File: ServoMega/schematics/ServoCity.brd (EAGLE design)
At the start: 108.9 x 55.9 mm, 2 parts

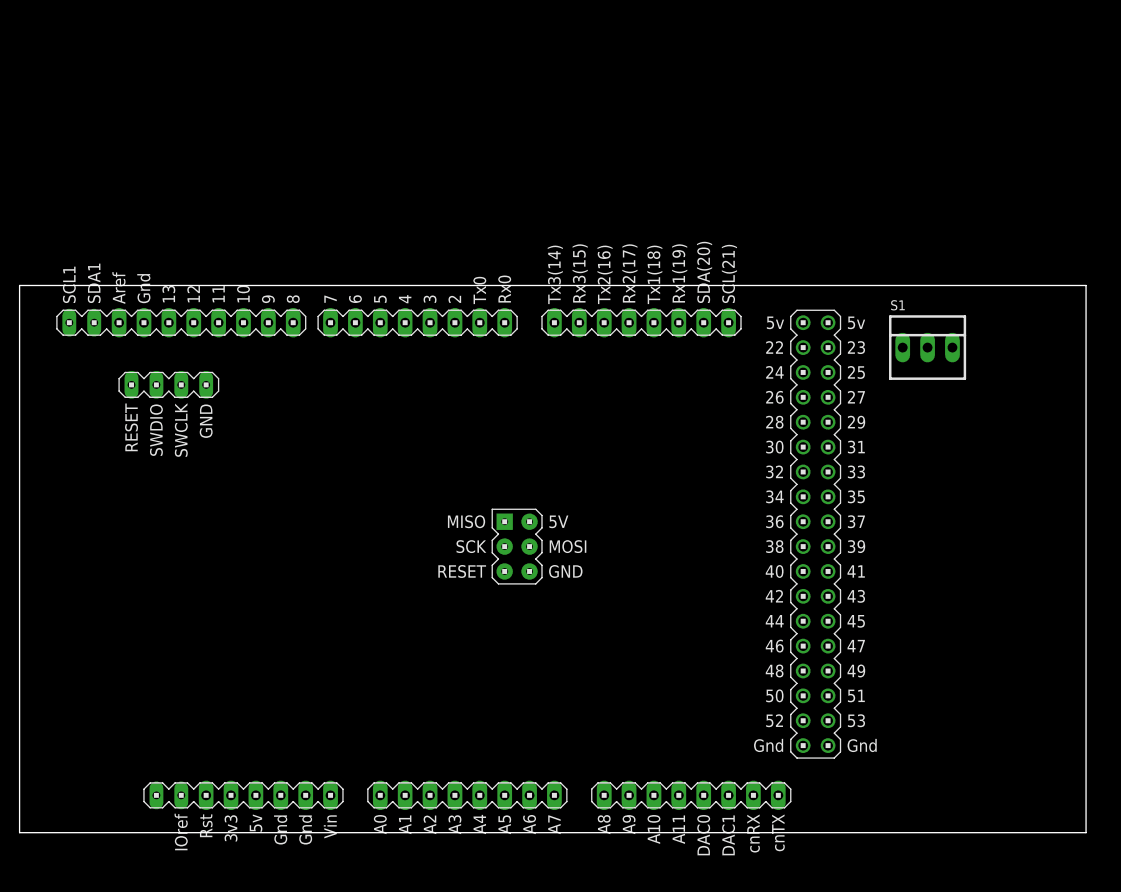
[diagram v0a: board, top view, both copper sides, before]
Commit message: HOK post laptop update
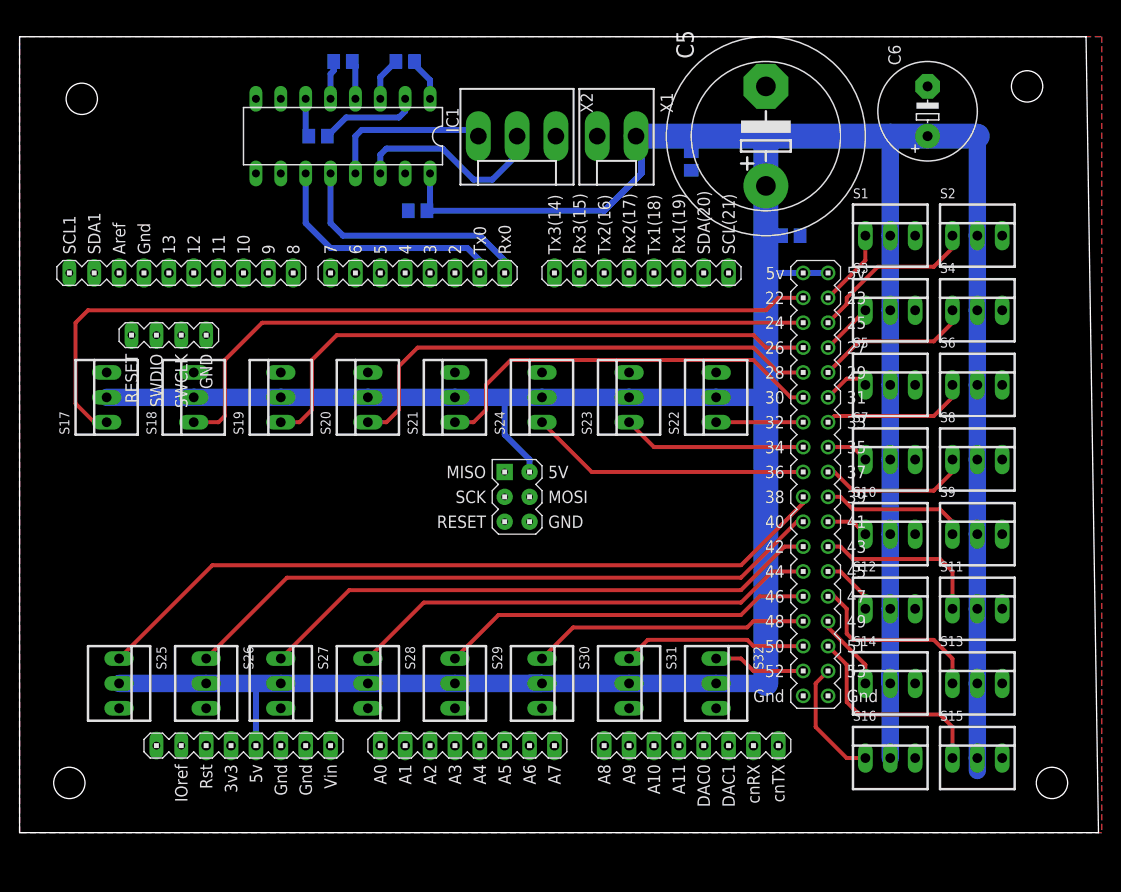
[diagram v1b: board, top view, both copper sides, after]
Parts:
- added C1, C2, C3, C4: (no value), rcl:C0805
- added C5: 2k2, rcl:EB20D
- added C6: 470, rcl:E5-10,5
- added C8, C9: (no value), eagle-ltspice:C0805
- added IC1: MAX232, maxim:DIL16
- added S10, S11, S12, S13, S14, S15, S16, S17, S18, S19, S2, S20, S21, S22, S23, S24, S25, S26, S27, S28, S29, S3, S30, S31, S32, S4, S5, S6, S7, S8, S9: 22-23-2031, con-molex:22-23-2031
- added X1: (no value), con-molex:KK-156-2
- added X2: (no value), con-molex:KK-156-3
- moved S1 12.0 mm to (88.9, 61.0)
- moved U$1 5.08 mm to (61.0, 26.7)
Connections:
- new net 5V: C5.+, C6.+, C8.1, C9.1, S1.2, S10.2, S11.2, S12.2, S13.2, S14.2, S15.2, S16.2, S17.2, S18.2, S19.2, S2.2, S20.2, S21.2, S22.2, S23.2, S24.2, S25.2, S26.2, S27.2, S28.2, S29.2, S3.2, S30.2, S31.2, S32.2, S4.2, S5.2, S6.2, S7.2, S8.2, S9.2, X1.1
- new net GND: C4.2, C5.-, C6.-, C8.2, C9.2, IC1.15, S1.3, S10.3, S11.3, S12.3, S13.3, S14.3, S15.3, S16.3, S17.3, S18.3, S19.3, S2.3, S20.3, S21.3, S22.3, S23.3, S24.3, S25.3, S26.3, S27.3, S28.3, S29.3, S3.3, S30.3, S31.3, S32.3, S4.3, S5.3, S6.3, S7.3, S8.3, S9.3, U$1.5V_ICSP, U$1.GND1, U$1.GND_1, U$1.GND_2, U$1.GND_A, U$1.GND_B, X1.2, X2.1
- new net N$1: IC1.14, X2.2
- new net N$2: IC1.13, X2.3
- new net N$3: C1.1, IC1.1
- new net N$4: C1.2, IC1.3
- new net N$5: C2.1, IC1.4
- new net N$6: C2.2, IC1.5
- new net N$7: C3.1, IC1.2
- new net N$8: C3.2, IC1.6
- new net RX: IC1.12, U$1.RX0
- new net SERVO1: S1.1, U$1.23
- new net SERVO10: S10.1, U$1.41
- new net SERVO11: S11.1, U$1.43
- new net SERVO12: S12.1, U$1.45
- new net SERVO13: S13.1, U$1.47
- new net SERVO14: S14.1, U$1.49
- new net SERVO15: S15.1, U$1.51
- new net SERVO16: S16.1, U$1.53
- new net SERVO17: S17.1, U$1.22
- new net SERVO18: S18.1, U$1.24
- new net SERVO19: S19.1, U$1.26
- new net SERVO2: S2.1, U$1.25
- new net SERVO20: S20.1, U$1.28
- new net SERVO21: S21.1, U$1.30
- new net SERVO22: S22.1, U$1.32
- new net SERVO23: S23.1, U$1.34
- new net SERVO24: S24.1, U$1.36
- new net SERVO25: S25.1, U$1.38
- new net SERVO26: S26.1, U$1.40
- new net SERVO27: S27.1, U$1.42
- new net SERVO28: S28.1, U$1.44
- new net SERVO29: S29.1, U$1.46
- new net SERVO3: S3.1, U$1.27
- new net SERVO30: S30.1, U$1.48
- new net SERVO31: S31.1, U$1.50
- new net SERVO32: S32.1, U$1.52
- new net SERVO4: S4.1, U$1.29
- new net SERVO5: S5.1, U$1.31
- new net SERVO6: S6.1, U$1.33
- new net SERVO7: S7.1, U$1.35
- new net SERVO8: S8.1, U$1.37
- new net SERVO9: S9.1, U$1.39
- new net TX: IC1.11, U$1.TX0
- new net VCC: C4.1, IC1.16, U$1.5V, U$1.5V_A, U$1.5V_B, U$1.GND_ICSP
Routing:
- net 5V: track 0.00 -> 367.3 mm
- net VCC: track 0.00 -> 199.9 mm
- net SERVO17: track 0.00 -> 87.6 mm
- net SERVO25: track 0.00 -> 77.1 mm
- net SERVO18: track 0.00 -> 69.8 mm
- net SERVO26: track 0.00 -> 66.7 mm
- net SERVO19: track 0.00 -> 60.5 mm
- net SERVO27: track 0.00 -> 58.1 mm
- net SERVO20: track 0.00 -> 51.3 mm
- net SERVO28: track 0.00 -> 48.1 mm
- net SERVO21: track 0.00 -> 41.3 mm
- net SERVO29: track 0.00 -> 38.2 mm
- net SERVO24: track 0.00 -> 28.8 mm
- net SERVO30: track 0.00 -> 28.2 mm
- net TX: track 0.00 -> 25.7 mm
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- added copper zone on layer 1, net GND
- added copper zone on layer 16, net GND
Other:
- board size 108.9 x 55.9 mm -> 110.2 x 81.3 mm
